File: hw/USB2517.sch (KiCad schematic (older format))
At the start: 45 parts, among them J1 EXT_PWR, J2 USB_C_Receptacle_USB2.0, U1 MIC5219-3.3, U2 LM1085-5.0, U3 USB2517, U4 24LC02, Y1 24Mhz

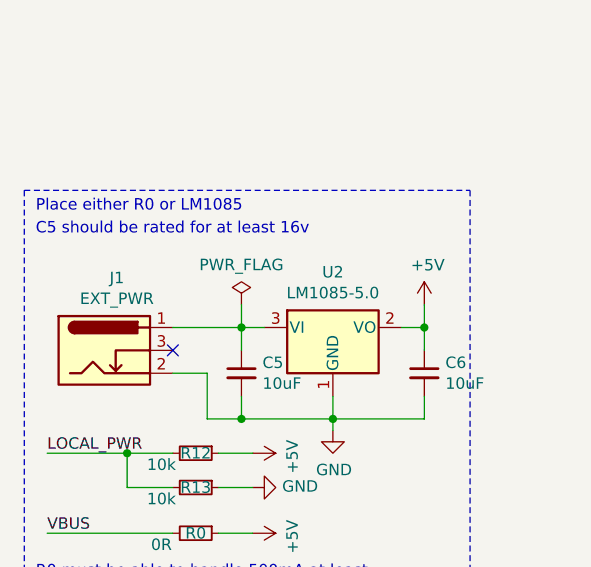
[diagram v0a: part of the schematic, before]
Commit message: Begin routing
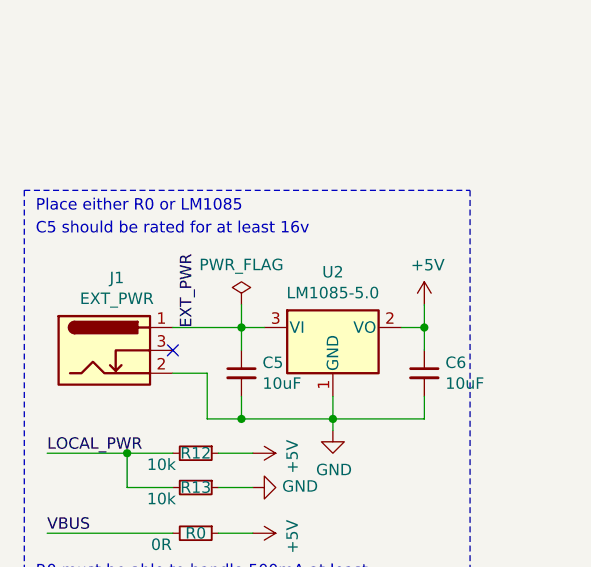
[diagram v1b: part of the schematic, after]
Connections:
- net EXT_PWR: now reaches C5.1, J1.1, U2.3 (VI)
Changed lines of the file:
@@
 	1600 3050 1450 3050
 NoConn ~ 1450 2950
+Text Label 1550 2850 1    50   ~ 0
+EXT_PWR
 $EndSCHEMATC
